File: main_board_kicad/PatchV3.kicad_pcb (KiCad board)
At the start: 4 copper layers, 100 x 50 mm, 94 parts, among them J1 Conn_02x04_Counter_Clockwise, J2 U.FL-R-SMT(01), J3 Conn_02x04_Odd_Even, J4 2908-05WB-MG, J5 JST PH SM4 S2B, J6 JST PH SM4 S2B, J7 JST PH SM4 S2B, U1 LoRa-E5, U2 INA2321EA_250, U3 OPA2349EA_250, U4 OPA2349EA_250, U5 SPV1050TTR, U6 LT3009IDCTRMPBF

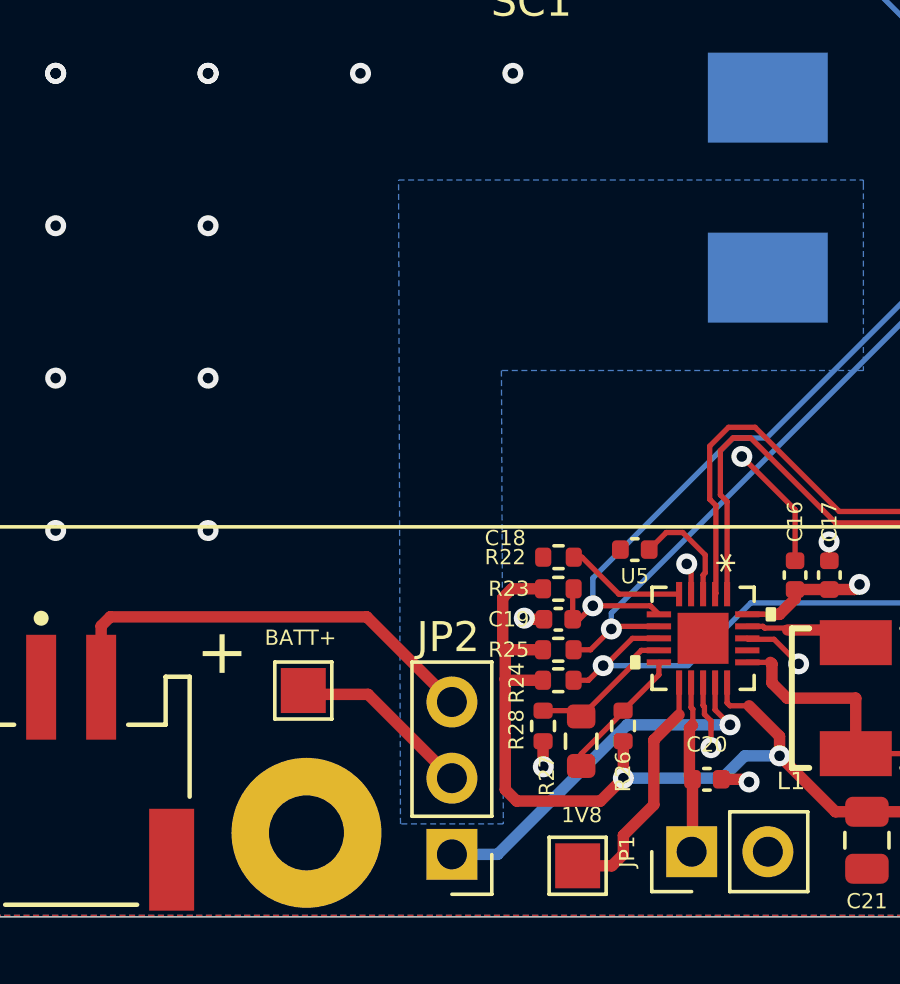
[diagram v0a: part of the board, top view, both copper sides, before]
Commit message: catchup
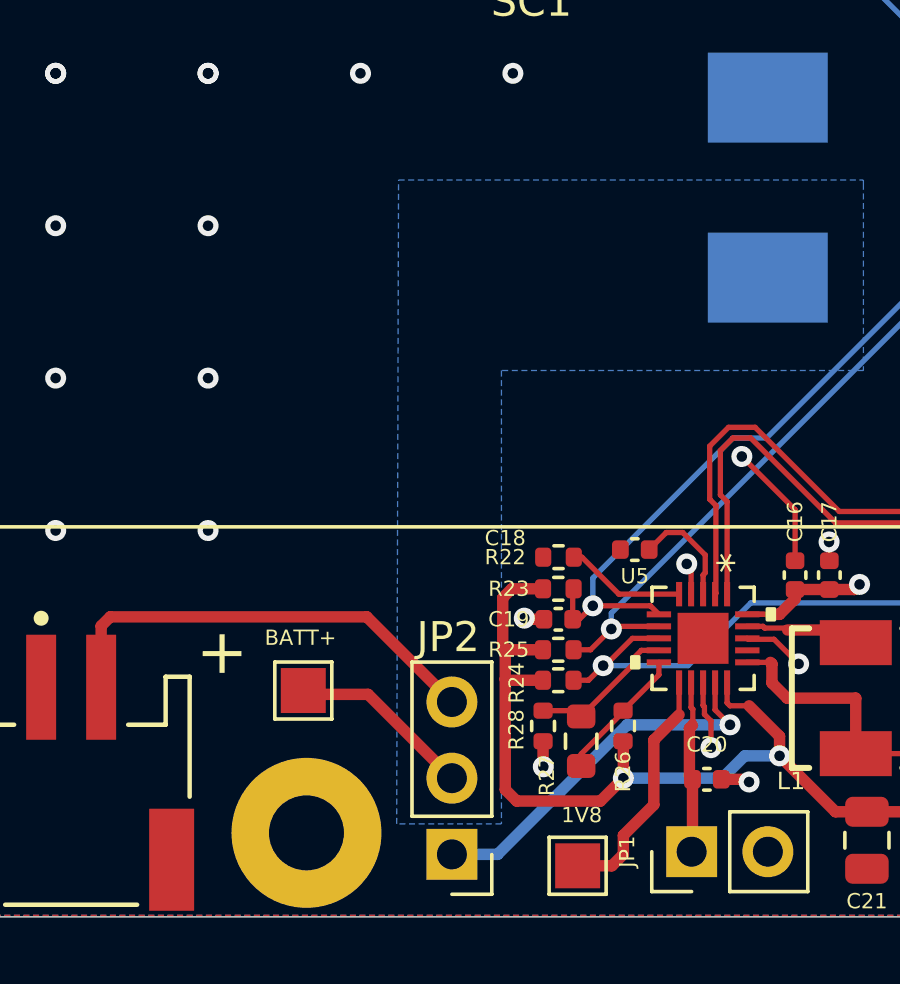
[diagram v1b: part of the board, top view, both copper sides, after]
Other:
- rule pad_to_mask_clearance: 0.051 -> 0
